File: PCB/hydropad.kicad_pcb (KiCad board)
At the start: 2 copper layers, 83.5 x 56 mm, 14 parts, among them SW1 SW_Push, SW2 SW_Push, SW3 SW_Push, SW4 SW_Push, SW5 SW_Push, SW6 RotaryEncoder_Switch, U1 MODULE-SEEEDUINO-XIAO

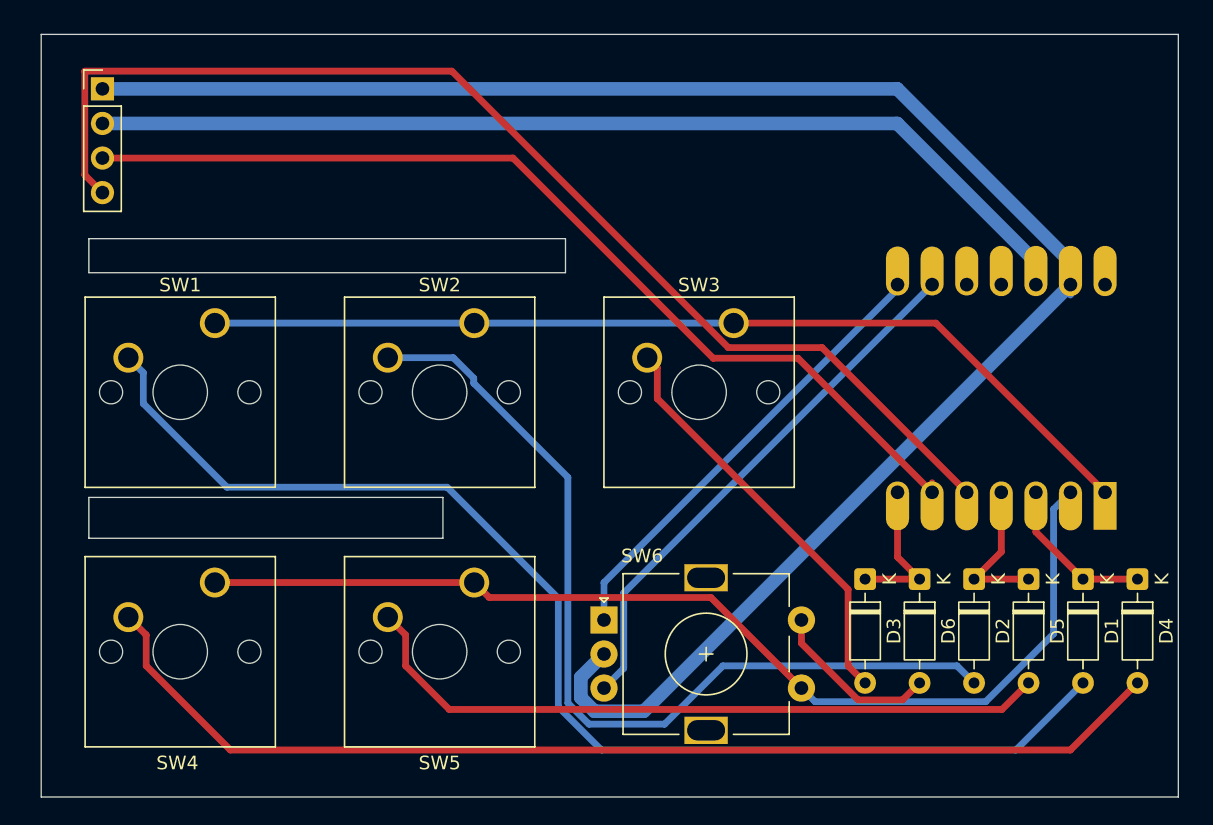
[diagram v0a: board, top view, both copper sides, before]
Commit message: Add some CAD data
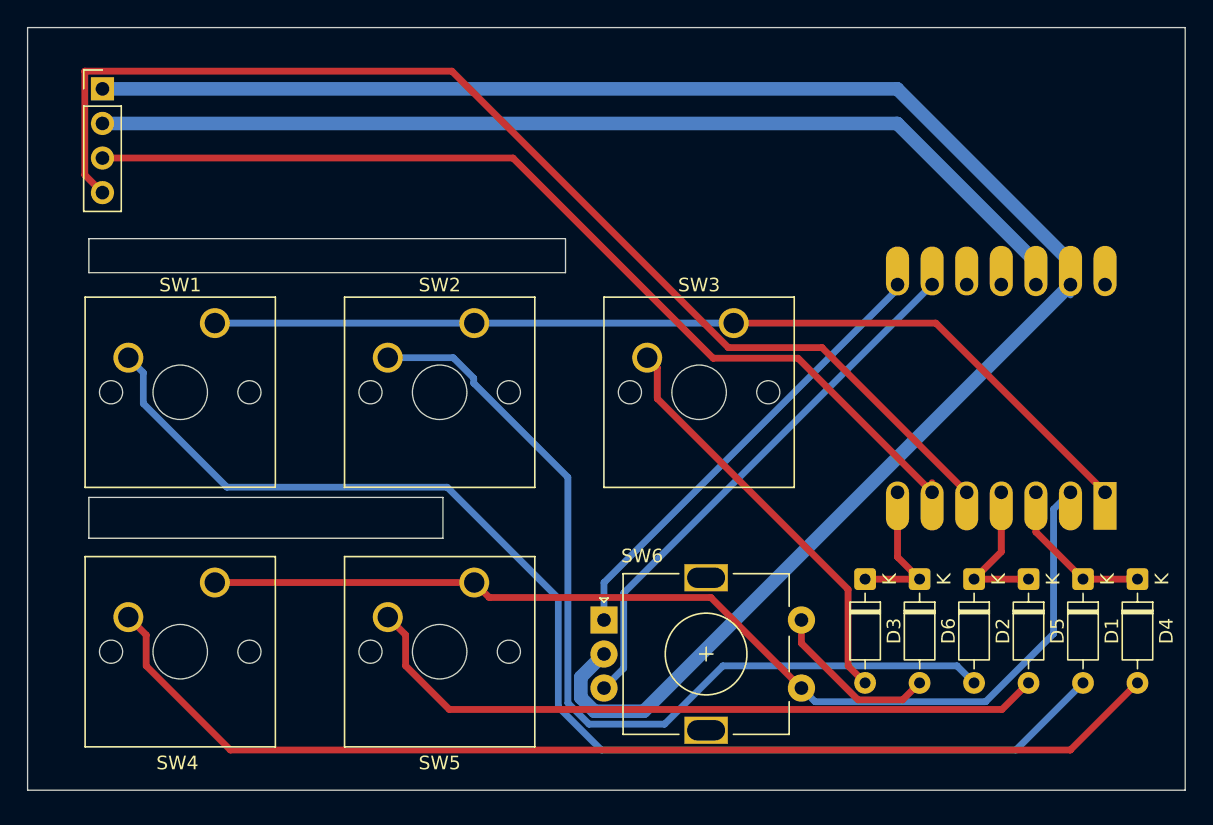
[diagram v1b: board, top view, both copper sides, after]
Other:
- board size 83.5 x 56 mm -> 85 x 56 mm
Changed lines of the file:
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@@
 	)
 	(gr_rect
-		(start 82.5 55)
-		(end 166 111)
+		(start 81.5 54.5)
+		(end 166.5 110.5)
 		(stroke
 			(width 0.05)
